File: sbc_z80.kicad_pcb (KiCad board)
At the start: 4 copper layers, 102.6 x 50.8 mm, 95 parts, among them J1 RC80 Bus, J2 CTC Header, J3 AVR-JTAG-10, J4 IDE, J5 PIO Header, J6 Port A, J7 Port B, J8 USB_B_Micro, Q1 IRLML6402, SW1 Reset, U1 DS1813R-5+T&R, U10 Z84C2010AEG, U11 74HCT273, U12 MAX40200AUK, U2 AP7381-33SA, U3 CPU -Z84C0020AEG, U4 CTC - Z84C3010AEG, U5 CPLD - EPM7032STC44, U6 SRAM - IS62C5128BL-45TLI, U7 74HCT2G04, U8 SST39SF040, U9 SIO/3 - Z84C4310AEG, X1 CTX-636 50mhz

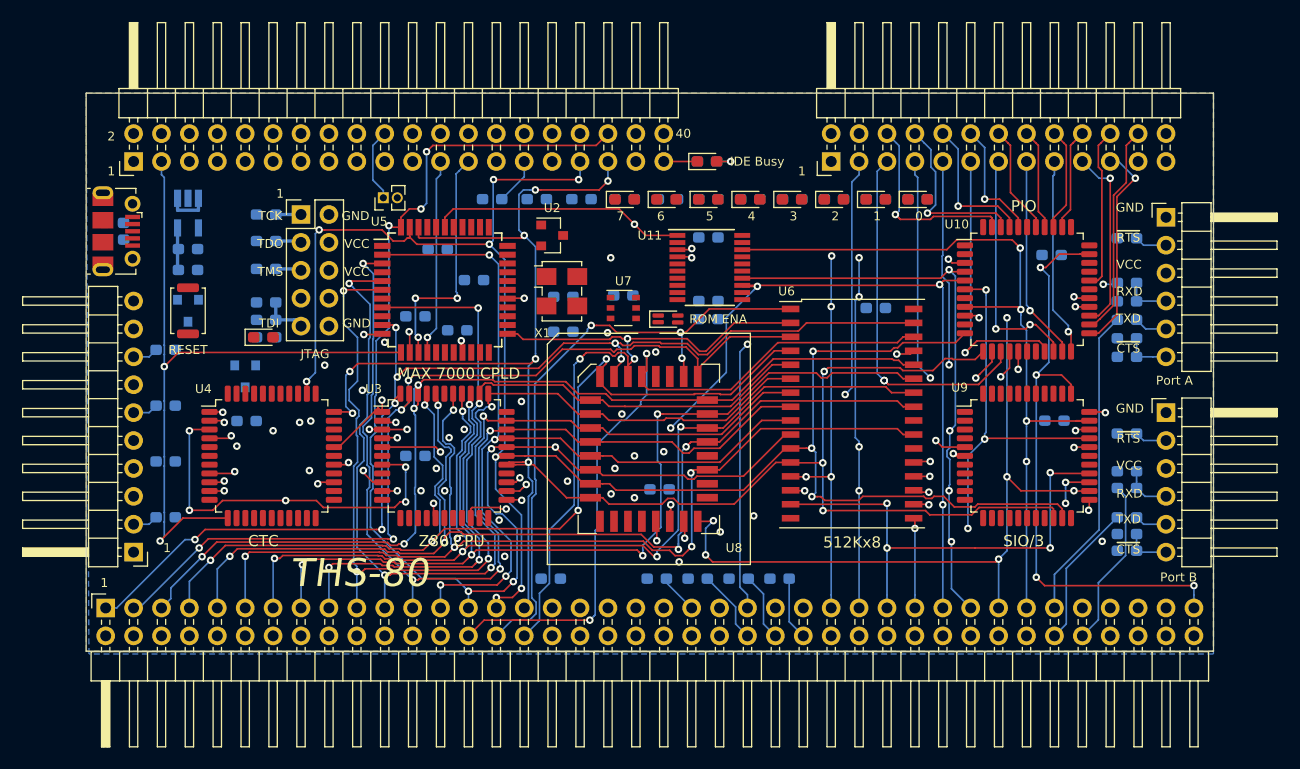
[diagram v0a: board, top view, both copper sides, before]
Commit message: checkpoint
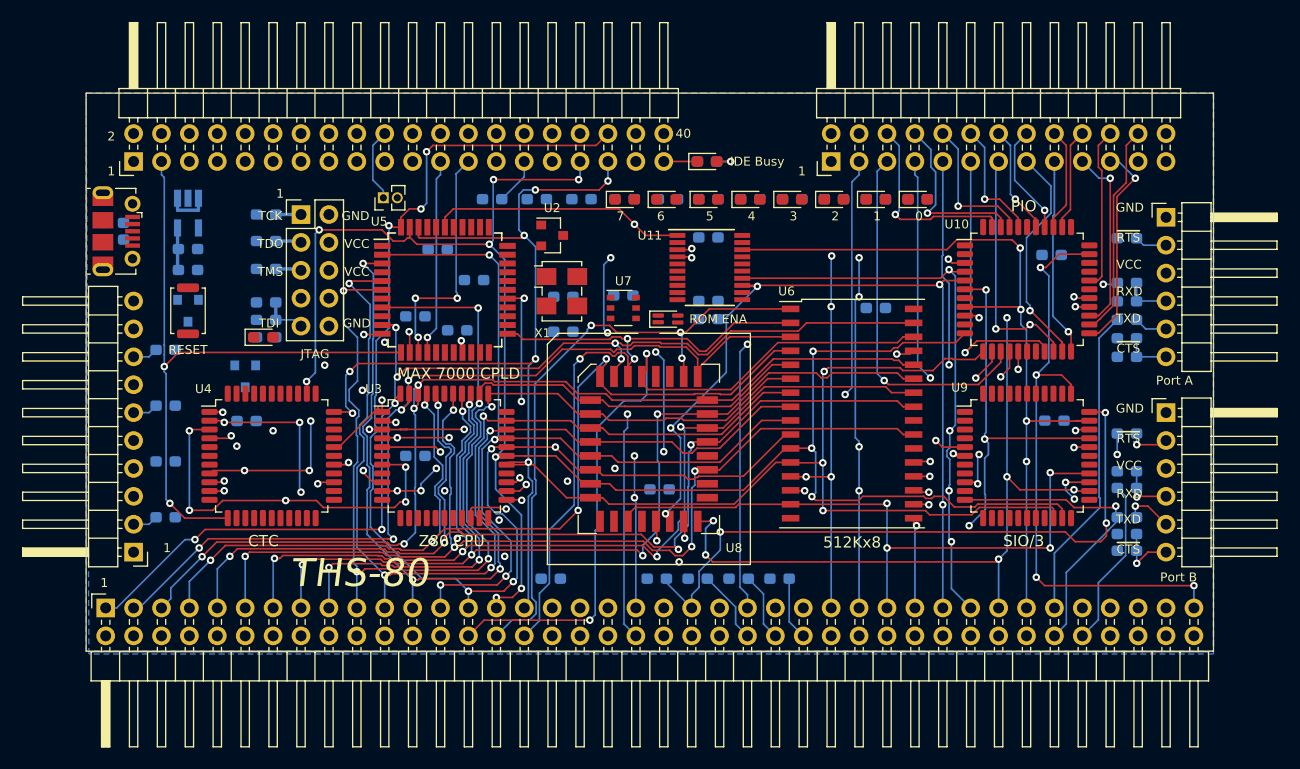
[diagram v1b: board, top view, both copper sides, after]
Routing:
- net /~IORQ: track 75.4 -> 0.00 mm, vias 3 -> 0
- net /~RTSB: track 0.00 -> 18.4 mm, vias 0 -> 3
- net /D2: track 110.4 -> 125.5 mm
- net /TXB: track 13.2 -> 27.8 mm, vias 0 -> 1
- net /~M1: track 114.5 -> 106.7 mm, vias 7 -> 6
- net /D7: track 145.9 -> 141.0 mm
- net /PA1: track 18.7 -> 20.5 mm
- net Net-(J7-Pad6): track 4.26 -> 5.92 mm, vias 0 -> 1
- net Net-(J7-Pad5): track 2.94 -> 4.38 mm, vias 0 -> 1
- net /PB2: track 9.20 -> 10.1 mm, vias 0 -> 1
- net /PB3: track 9.92 -> 10.8 mm, vias 0 -> 1
- net /TDI: track 4.12 -> 3.32 mm
- net /~ASTB: track 19.3 -> 18.5 mm
- net /D4: track 170.8 -> 171.6 mm
- net /A0: track 167.6 -> 166.9 mm
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- added copper zone on In2.Cu, net (none)
- removed copper zone on In2.Cu, net VCC
